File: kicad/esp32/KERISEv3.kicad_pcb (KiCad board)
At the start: 2 copper layers, 49 x 42 mm, 118 parts, among them P1 ANT, P10 PR_Slave, P11 PR_Host, P12 PR_Slave, P13 ENC_Host, P14 ENC_Slave, P15 ENC_Host, P16 ENC_Slave, P17 UART, P18 Fan, P2 Motor_L, P3 Motor_R, P4 Battery, P5 PR_Host, P6 PR_Slave, P7 PR_Host, P8 PR_Slave, P9 PR_Host, Q1 IRFML8244, Q2 IRFML8244, Q3 IRFML8244, Q4 IRFML8244, Q5 BSS138, Q6 IRFML8244, SW1 RESET, SW2 SW_PUSH_SMALL, U1 ESP32, U10 MPU6500, U11 AS5145, U12 AS5145, U2 XTAL, U3 FLASH, U4 DRV8835, U5 NJM2884, U6 AD8601, U7 AD8601, U8 AD8601, U9 AD8601

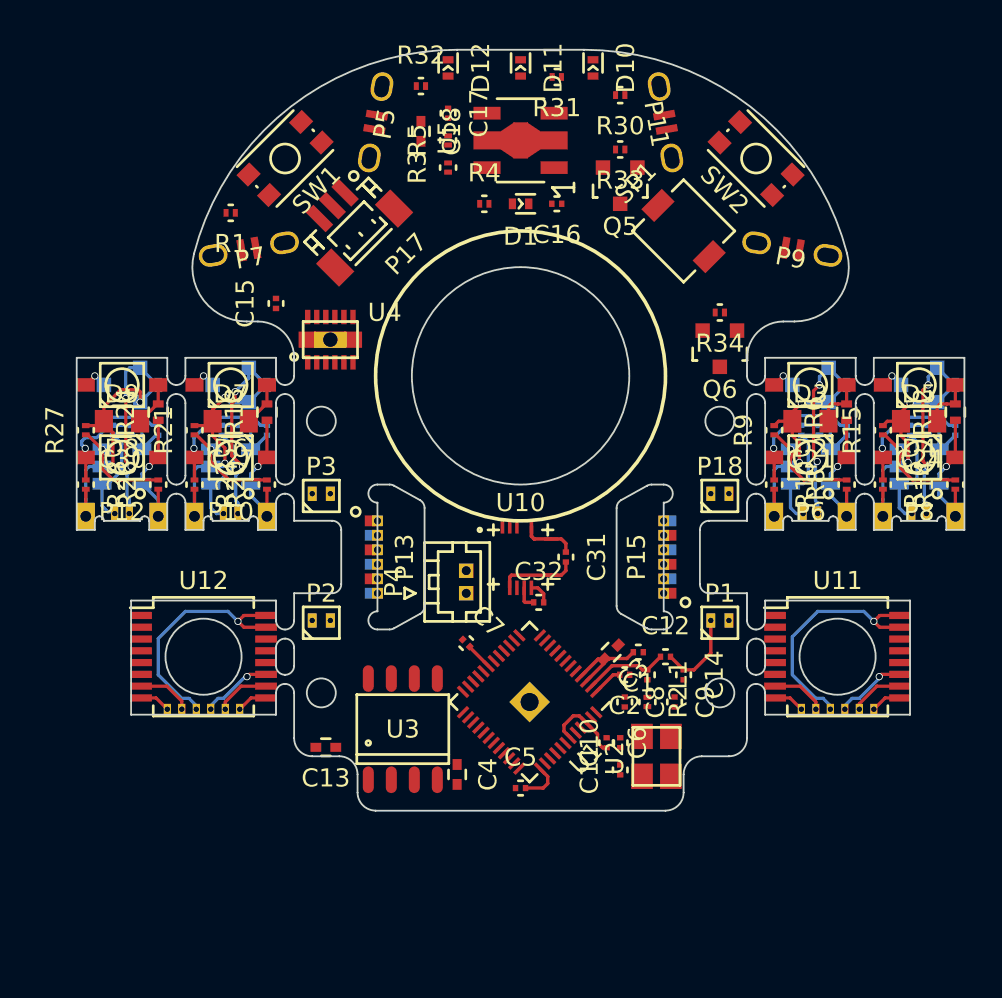
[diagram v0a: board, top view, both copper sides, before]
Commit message: 自動配線成功
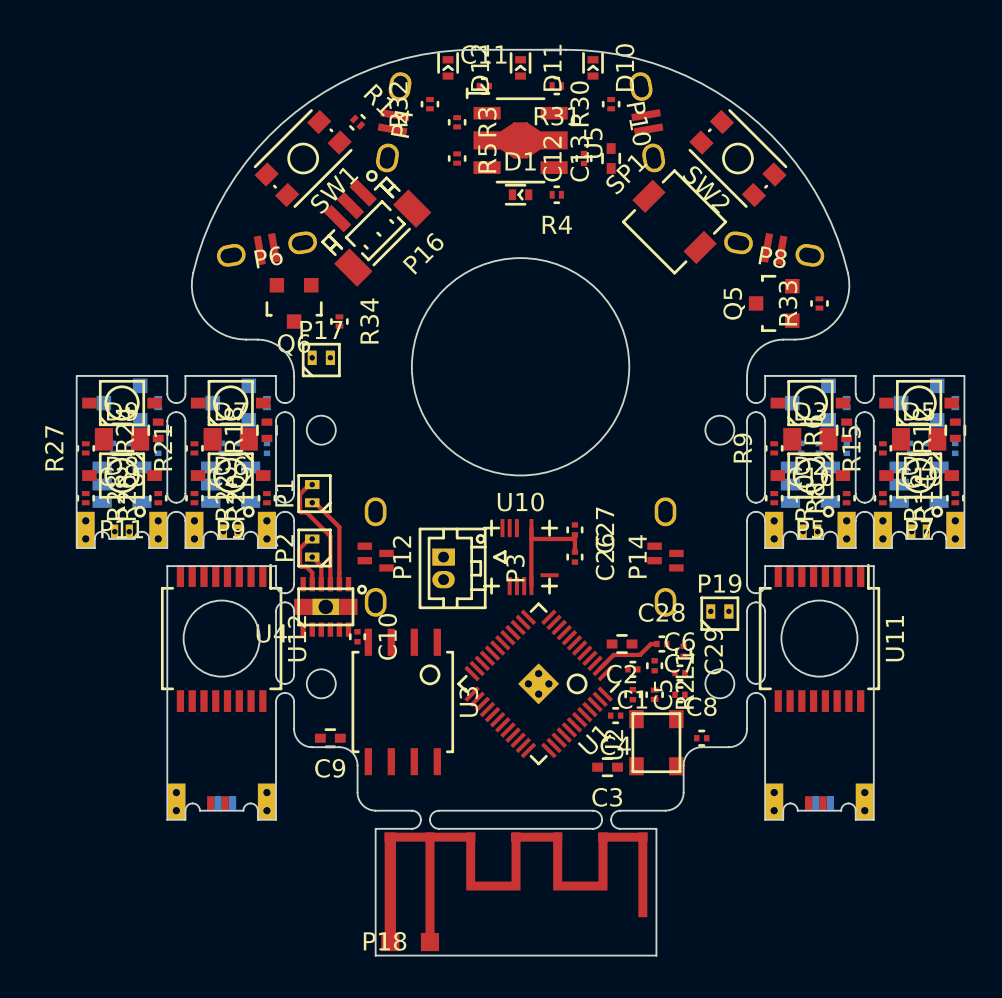
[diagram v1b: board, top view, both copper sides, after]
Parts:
- removed the C14 at (157.5, 119.5)
- removed the C15 at (135.0, 99.0)
- removed the C16 at (150.5, 93.5)
- removed the C17 at (144.5, 88.5)
- removed the C18 at (143.0, 89.5)
- removed the C5 at (148.5, 125.8)
- removed the C6 at (153.2, 123.2)
- removed the P15 at (156.4, 113.0)
- removed the P4 at (145.5, 115.0)
- added C13: 4.7u, Capacitors_SMD:C_0402, F.Cu at (153.5, 91.0)
- added C28: 4.7p, Capacitors_SMD:C_0201, F.Cu at (156.3, 117.8)
- added C29: 2.4p, Capacitors_SMD:C_0201, F.Cu at (157.5, 118.2)
- added C8: 22p, Capacitors_SMD:C_0201, F.Cu at (158.5, 123.0)
- added P14: ENC_Host, mouse:STAND_AS_HOST, F.Cu at (156.5, 113.0)
- added P16: UART, Connectors_JST:JST_SH_BM03B-SRSS-TB_03x1.00mm_Straight, F.Cu at (140.0, 94.5)
- added P19: ANT_Host, mouse:SMD_conn_2, F.Cu at (159.5, 116.0)
- C10: value 22p -> 0.1u
- C11: value 22p -> 0.33u
- C12: value 3.9p -> 0.1u
- C2: value 0.1u -> 10u; footprint Capacitors_SMD:C_0201 -> Capacitors_SMD:C_0402
- C4: value 10u -> 0.1u; footprint Capacitors_SMD:C_0402 -> Capacitors_SMD:C_0201
- C5: renamed from C8; value 3300p -> 3.3n
- C7: value 0.1u -> 22p
- L1: value 2.7n -> 2.4n
- P1: value ANT -> Motor_L
- P17: value UART -> Fan; footprint Connectors_JST:JST_SH_BM03B-SRSS-TB_03x1.00mm_Straight -> mouse:SMD_conn_2
- P18: value Fan -> PCB_ANT; footprint mouse:SMD_conn_2 -> mouse:ANT
- P2: value Motor_L -> Motor_R
- P3: value Motor_R -> Battery; footprint mouse:SMD_conn_2 -> Connectors_Hirose:Hirose_DF13-02P-1.25DSA_02x1.25mm_Straight
- U1: footprint mouse:UQFN-48-1EP_6x6mm_Pitch0.4mm -> mouse:ESP32
- U2: footprint Crystals:crystal_FA238-TSX3225 -> mouse:crystal_FA238-TSX3225
- U3: footprint Power_Integrations:SO-8 -> mouse:SOIJ-8_5.3x5.3mm_Pitch1.27mm
- moved C11 38.5 mm to (146.5, 87.0), turned to 0 degrees
- moved P18 30.5 mm to (141.0, 133.8)
- moved C12 27.9 mm to (152.0, 91.0), turned to 90 degrees
- moved Q6 23.6 mm to (136.0, 99.0)
- moved P1 23.6 mm to (137.0, 109.5), turned to 90 degrees
- moved R34 21.0 mm to (138.5, 100.0), turned to 270 degrees
- moved C10 15.6 mm to (139.5, 117.4), turned to 270 degrees
- moved U4 14.8 mm to (137.8, 115.8), turned to 180 degrees
- moved R33 13.9 mm to (165.0, 99.0), turned to 90 degrees
- moved C7 12.1 mm to (157.3, 120.6), turned to 0 degrees
- moved Q5 10.7 mm to (162.5, 99.0), turned to 90 degrees
- moved C4 9.33 mm to (153.8, 121.8), turned to 180 degrees
- moved R1 8.60 mm to (139.5, 89.0), turned to 315 degrees
- moved P17 7.65 mm to (137.5, 102.0), turned to 0 degrees
- moved P3 7.60 mm to (144.2, 113.0), turned to 270 degrees
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- renumbered C19 to C14, C20 to C15, C21 to C16, C22 to C17, C23 to C18, C24 to C19, C25 to C20, C26 to C21, C27 to C22, C28 to C23, C29 to C24, C30 to C25, C31 to C26, C32 to C27, C9 to C6, C13 to C9, P11 to P10, P12 to P11, P13 to P12, P14 to P13, P16 to P15, P5 to P4, P6 to P5, P7 to P6, P8 to P7, P9 to P8, P10 to P9
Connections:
- C10 pad 1: Net-(C10-Pad1) -> +3V3
- C11 pad 1: Net-(C11-Pad1) -> +BATT
- C12 pad 1: ANT -> +3V3
- C12 pad 2: Net-(C12-Pad2) -> GND
- C7 pad 1: GND -> Net-(C7-Pad1)
- C7 pad 2: +3V3 -> GND
- P1 pad 1: Net-(C12-Pad2) -> /Motor/MT_OUT_L1
- P1 pad 2: GND -> /Motor/MT_OUT_L2
- P12 pad 1: /ENC_L/MISO -> +3V3
- P12 pad 3: ENC_~CS -> GND
- P12 pad 4: +3V3 -> /ENC_L/MISO
- P12 pad 5: GND -> ENC_~CS
- P13 pad 1: /ENC_L/s_MISO -> /ENC_L/s_3.3V
- P13 pad 3: /ENC_L/s_CSn -> /ENC_L/s_MOSI
- P13 pad 4: /ENC_L/s_3.3V -> /ENC_L/s_MISO
- P13 pad 5: /ENC_L/s_VSS -> /ENC_L/s_CSn
- P13 pad 6: /ENC_L/s_MOSI -> /ENC_L/s_VSS
- P15 pad 1: /ENC_R/s_MISO -> /ENC_R/s_3.3V
- P15 pad 3: /ENC_R/s_CSn -> /ENC_R/s_MOSI
- P15 pad 4: /ENC_R/s_3.3V -> /ENC_R/s_MISO
- P15 pad 5: /ENC_R/s_VSS -> /ENC_R/s_CSn
- P15 pad 6: /ENC_R/s_MOSI -> /ENC_R/s_VSS
- P17 pad 1: GND -> +BATT
- P17 pad 2: UART-RX -> /Fan/fan_to_fet
- P18 pad 1: +BATT -> (no net)
- P18 pad 2: /Fan/fan_to_fet -> (no net)
- P2 pad 1: /Motor/MT_OUT_L1 -> /Motor/MT_OUT_R1
- P2 pad 2: /Motor/MT_OUT_L2 -> /Motor/MT_OUT_R2
- P3 pad 1: /Motor/MT_OUT_R1 -> +BATT
- P3 pad 2: /Motor/MT_OUT_R2 -> GND
- U1 pad 44: Net-(C11-Pad1) -> Net-(C8-Pad1)
- U1 pad 45: Net-(C10-Pad1) -> Net-(C7-Pad1)
- U2 pad 1: Net-(C11-Pad1) -> Net-(C8-Pad1)
- U2 pad 2: Net-(C10-Pad1) -> Net-(C7-Pad1)
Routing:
- net +3V3: track 20.2 -> 0.00 mm
- net /IR_RCV_SR/s_GND: track 14.5 -> 0.00 mm, vias 2 -> 0
- net /IR_RCV_FR/s_GND: track 14.0 -> 0.00 mm, vias 2 -> 0
- net /ENC_R/s_3.3V: track 13.6 -> 0.00 mm, vias 1 -> 0
- net /ENC_L/s_3.3V: track 13.6 -> 0.00 mm, vias 1 -> 0
- net /IR_RCV_SL/s_GND: track 13.2 -> 0.00 mm, vias 2 -> 0
- net /IR_RCV_FL/s_GND: track 13.2 -> 0.00 mm, vias 2 -> 0
- net /IR_RCV_FR/s_IR_LED: track 10.2 -> 0.00 mm, vias 2 -> 0
- net /IR_RCV_SR/s_IR_LED: track 10.2 -> 0.00 mm, vias 2 -> 0
- net /IR_RCV_FL/s_IR_LED: track 9.93 -> 0.00 mm, vias 2 -> 0
- net /IR_RCV_SL/s_IR_LED: track 9.85 -> 0.00 mm, vias 2 -> 0
- net Net-(C24-Pad2): track 7.56 -> 0.00 mm, vias 1 -> 0
- net /IR_RCV_SR/s_3.3V: track 7.54 -> 0.00 mm, vias 1 -> 0
- net /IR_RCV_SL/s_3.3V: track 7.54 -> 0.00 mm, vias 1 -> 0
- net /IR_RCV_FR/s_3.3V: track 7.54 -> 0.00 mm, vias 1 -> 0
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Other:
- board size 49 x 42 mm -> 49 x 50 mm
- net class 3.3V: clearance 0.2 -> 0.16; trace_width 0.29 -> 0.238; via_dia 0.4 -> 0.36
- net class BATT: clearance 0.2 -> 0.16; trace_width 0.29 -> 0.32; via_dia 0.4 -> 0.36
- net class Default: clearance 0.2 -> 0.16; trace_width 0.19 -> 0.18; via_dia 0.4 -> 0.36
- net class GND: clearance 0.2 -> 0.16; trace_width 0.29 -> 0.32; via_dia 0.4 -> 0.36
- net class LED added: clearance 0.16, trace_width 0.3, via_dia 0.36, via_drill 0.3
- net class Motor: clearance 0.2 -> 0.16; trace_width 0.29 -> 0.3; via_dia 0.4 -> 0.36
- rule trace_clearance: 0.2 -> 0.16
- rule via_min_size: 0.4 -> 0.36

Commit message: 更新
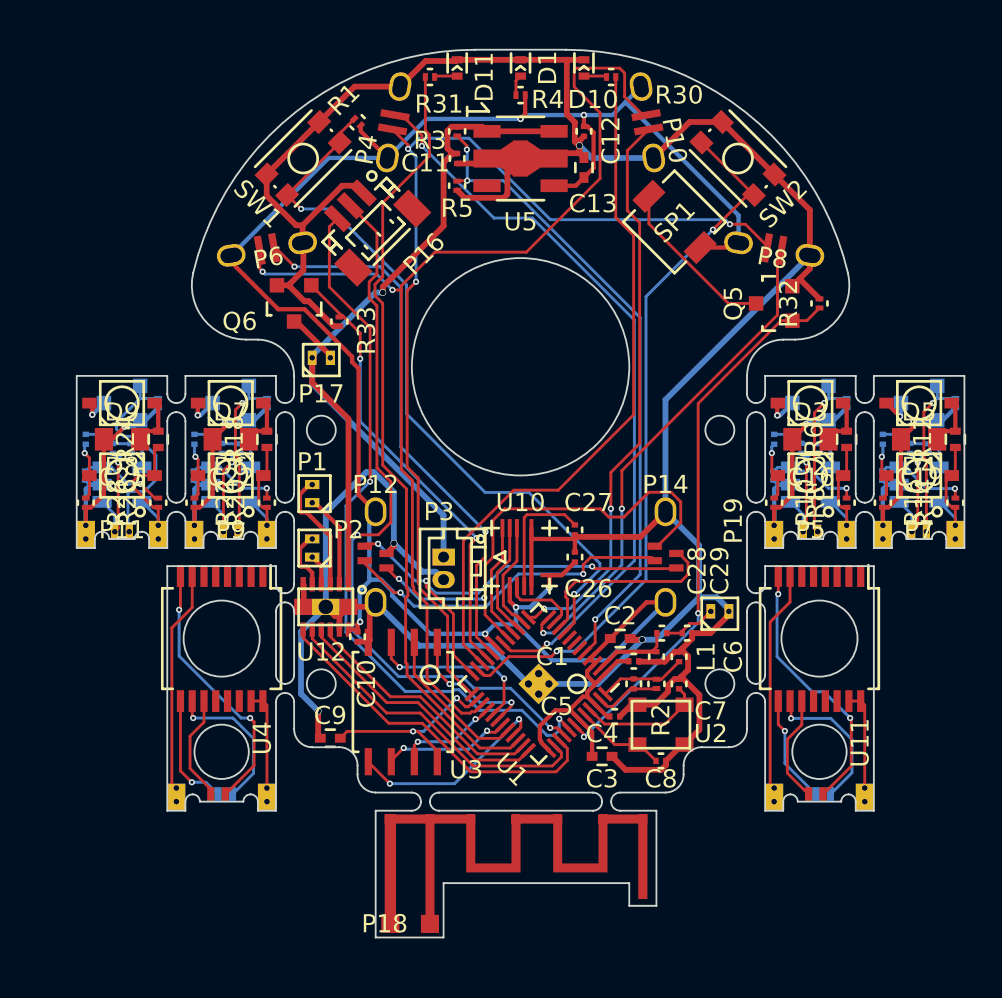
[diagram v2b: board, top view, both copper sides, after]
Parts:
- removed D12: LED, LEDs:LED_0402
- removed the R32 at (143.5, 88.0)
- R15, R21, R27, R9: moved to B.Cu
- moved R31 7.02 mm to (143.5, 86.5), turned to 0 degrees
- moved D1 7.00 mm to (148.5, 86.0), turned to 270 degrees
- moved R4 5.85 mm to (148.5, 87.5)
- moved C11 4.27 mm to (145.0, 91.0), turned to 270 degrees
- moved C15 4.03 mm to (162.5, 106.5), turned to 270 degrees
- moved C18 4.03 mm to (168.5, 106.5), turned to 270 degrees
- moved C21 4.03 mm to (130.5, 106.5), turned to 270 degrees
- moved C24 4.03 mm to (124.5, 106.5), turned to 270 degrees
- moved D11 3.50 mm to (145.0, 86.0)
- moved C8 2.57 mm to (156.2, 124.2)
- moved C13 1.58 mm to (152.0, 91.5)
- moved C12 1.50 mm to (152.0, 89.5), turned to 270 degrees
- moved R15 1.50 mm to (168.5, 108.5), turned to 270 degrees
- moved R21 1.50 mm to (130.5, 108.5), turned to 270 degrees
- moved R27 1.50 mm to (124.5, 108.5), turned to 270 degrees
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- renumbered R33 to R32, R34 to R33
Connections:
- net RESET renamed Net-(R1-Pad1)
- U1 pad 10: PR-RCV-SL -> ENC_MISO
- U1 pad 11: PR-RCV-FL -> AXIS_MISO
- U1 pad 12: BAT-VOL -> PR-RCV-FR
- U1 pad 13: AXIS_MISO -> PR-RCV-SR
- U1 pad 17: ENC_SCK -> ENC_~CS
- U1 pad 18: PR-LED-FR -> PR-RCV-SL
- U1 pad 20: PR-LED-FL -> PR-RCV-FL
- U1 pad 21: ENC_MISO -> FAN
- U1 pad 24: LED_2 -> ENC_SCK
- U1 pad 25: MT-IN-L1 -> PR-LED-FR
- U1 pad 27: MT-IN-L2 -> PR-LED-FL
- U1 pad 34: LED_3 -> LED_2
- U1 pad 35: MT-IN-R1 -> MT-IN-L1
- U1 pad 36: ENC_~CS -> MT-IN-L2
- U1 pad 38: MT-IN-R2 -> MT-IN-R1
- U1 pad 39: FAN -> MT-IN-R2
- U1 pad 5: PR-RCV-FR -> BAT-VOL
- U1 pad 8: PR-RCV-SR -> (no net)
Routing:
- net GND: track 6.55 -> 194.7 mm, vias 0 -> 4
- net +3V3: track 0.00 -> 122.9 mm, vias 0 -> 6
- net PR-LED-FL: track 0.00 -> 61.5 mm, vias 0 -> 2
- net PR-LED-FR: track 0.00 -> 56.0 mm, vias 0 -> 3
- net +BATT: track 0.00 -> 49.8 mm, vias 0 -> 1
- net LED_2: track 0.00 -> 43.2 mm
- net PR-RCV-SL: track 0.00 -> 41.0 mm, vias 0 -> 2
- net UART-RX: track 0.00 -> 40.4 mm, vias 0 -> 2
- net UART-TX: track 0.00 -> 40.3 mm, vias 0 -> 2
- net Net-(R1-Pad1): track 0.00 -> 40.3 mm, vias 0 -> 2
- net BUTTON: track 0.00 -> 39.6 mm, vias 0 -> 2
- net LED_1: track 0.00 -> 38.5 mm
- net BAT-VOL: track 0.00 -> 35.7 mm, vias 0 -> 3
- net PR-RCV-SR: track 0.00 -> 31.3 mm, vias 0 -> 2
- net SPEAKER: track 0.00 -> 30.8 mm, vias 0 -> 2
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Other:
- board size 49 x 50 mm -> 49 x 49 mm
- net class BATT: via_dia 0.36 -> 0.38; via_drill 0.3 -> 0.32
- net class Default: trace_width 0.18 -> 0.16; via_dia 0.36 -> 0.34
- net class GND: via_dia 0.36 -> 0.38; via_drill 0.3 -> 0.32
- net class LED: trace_width 0.3 -> 0.24
- rule trace_min: 0.18 -> 0.16
- rule via_min_size: 0.36 -> 0.34
